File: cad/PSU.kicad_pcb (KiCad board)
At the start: 2 copper layers, 94 x 63.5 mm, 20 parts, among them J1 Input, J2 Barrel_Jack_Switch, J3 Output, J4 INA219 breakout, J5 WWG-A, J6 WWG-B, Q1 LM317T, U1 LM7805_TO220, U2 X9C103P

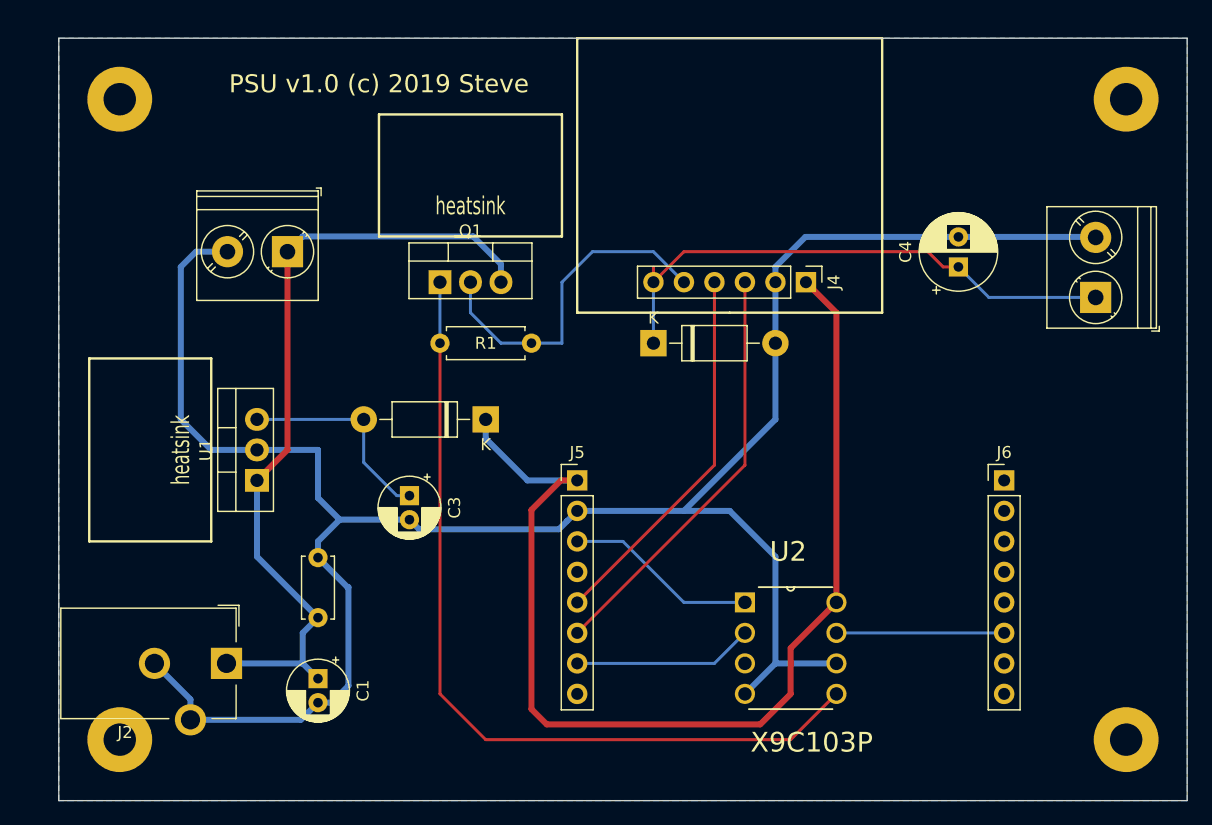
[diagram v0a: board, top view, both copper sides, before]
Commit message: layout again
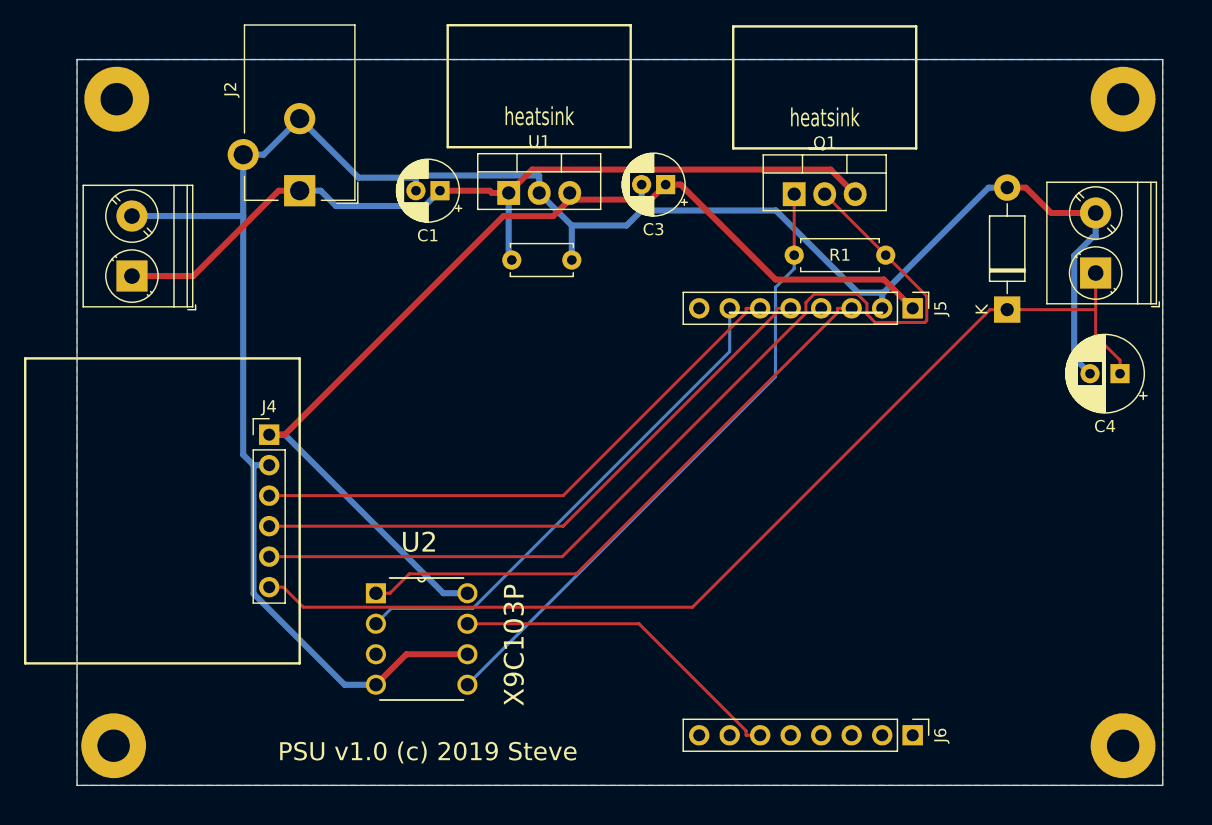
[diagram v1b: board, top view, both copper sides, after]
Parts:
- removed D1: 1N4001, Diode_THT:D_DO-41_SOD81_P10.16mm_Horizontal
- removed REF** (x4): MountingHole_2.7mm_M2.5_Pad, MountingHole:MountingHole_2.7mm_M2.5_Pad
- added REF1: MountingHole_2.7mm_M2.5_Pad, MountingHole:MountingHole_2.7mm_M2.5_Pad, F.Cu at (42.9, 36.8)
- added REF2: MountingHole_2.7mm_M2.5_Pad, MountingHole:MountingHole_2.7mm_M2.5_Pad, F.Cu at (42.7, 90.7)
- added REF3: MountingHole_2.7mm_M2.5_Pad, MountingHole:MountingHole_2.7mm_M2.5_Pad, F.Cu at (126.7, 90.7)
- added REF4: MountingHole_2.7mm_M2.5_Pad, MountingHole:MountingHole_2.7mm_M2.5_Pad, F.Cu at (126.7, 36.8)
- J5: value WWG-A -> WWG left
- J6: value WWG-B -> WWG right
- moved J4 46.5 mm to (55.6, 64.8), turned to 0 degrees
- moved C1 41.9 mm to (69.8, 44.5), turned to 180 degrees
- moved J2 39.8 mm to (58.2, 44.5), turned to 180 degrees
- moved C2 33.9 mm to (75.8, 50.2), turned to 0 degrees
- moved C3 33.6 mm to (88.6, 43.9), turned to 180 degrees
- moved U1 31.8 mm to (75.6, 44.6), turned to 0 degrees
- moved J5 31.4 mm to (109.2, 54.2), turned to 270 degrees
- moved U2 30.7 mm to (72.1, 85.6)
- moved Q1 30.4 mm to (99.4, 44.7)
- moved R1 30.4 mm to (107.0, 49.8)
- moved D2 29.6 mm to (117.1, 54.4), turned to 90 degrees
- moved J6 22.6 mm to (109.2, 89.8), turned to 270 degrees
- moved C4 16.1 mm to (126.5, 59.7), turned to 180 degrees
- moved J1 13.1 mm to (44.2, 51.6), turned to 90 degrees
- moved J3 2.03 mm to (124.5, 51.3)
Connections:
- C3 pad 1: Net-(C3-Pad1) -> +5V
- U1 pad 3: Net-(C3-Pad1) -> +5V
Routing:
- net Net-(J4-Pad5): track 28.6 -> 79.9 mm
- net Net-(C4-Pad1): track 45.8 -> 89.0 mm
- net Net-(J5-Pad3): track 16.1 -> 49.7 mm
- net Net-(J5-Pad7): track 15.0 -> 42.5 mm
- net Net-(J4-Pad4): track 31.4 -> 51.2 mm
- net Net-(Q1-Pad1): track 70.5 -> 52.1 mm
- net Net-(C3-Pad1): track 17.4 -> 0.00 mm
- net Net-(J6-Pad6): track 14.0 -> 28.4 mm
- net Net-(J4-Pad3): track 35.0 -> 47.6 mm
- net +15V: track 66.9 -> 71.7 mm
- net GND: track 179.7 -> 176.5 mm
- net +5V: track 92.2 -> 89.0 mm
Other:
- board size 94 x 63.5 mm -> 90.4 x 60.5 mm
